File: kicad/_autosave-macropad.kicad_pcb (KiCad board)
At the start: 2 copper layers, 102 x 92 mm, 16 parts, among them J1 Conn_01x04_Socket, SW1 Kailh Choc, SW10 RotaryEncoder_Switch, SW11 RotaryEncoder_Switch, SW12 SW_Push, SW2 Kailh Choc, SW3 Kailh Choc, SW4 Kailh Choc, SW5 CherryMX, SW6 Kailh Choc, SW7 Kailh Choc, SW8 Kailh Choc, SW9 Kailh Choc, U1 Pico, U2 SKQUCAA010

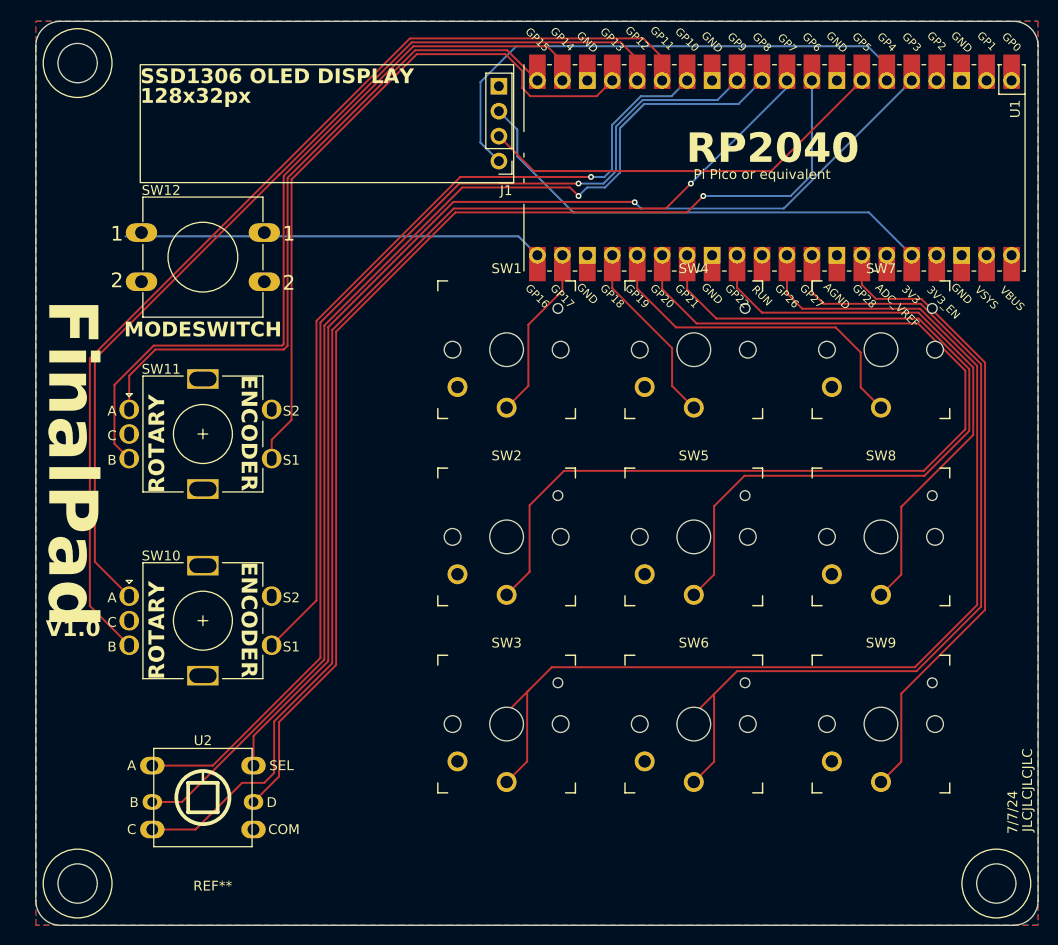
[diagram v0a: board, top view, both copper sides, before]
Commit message: updated
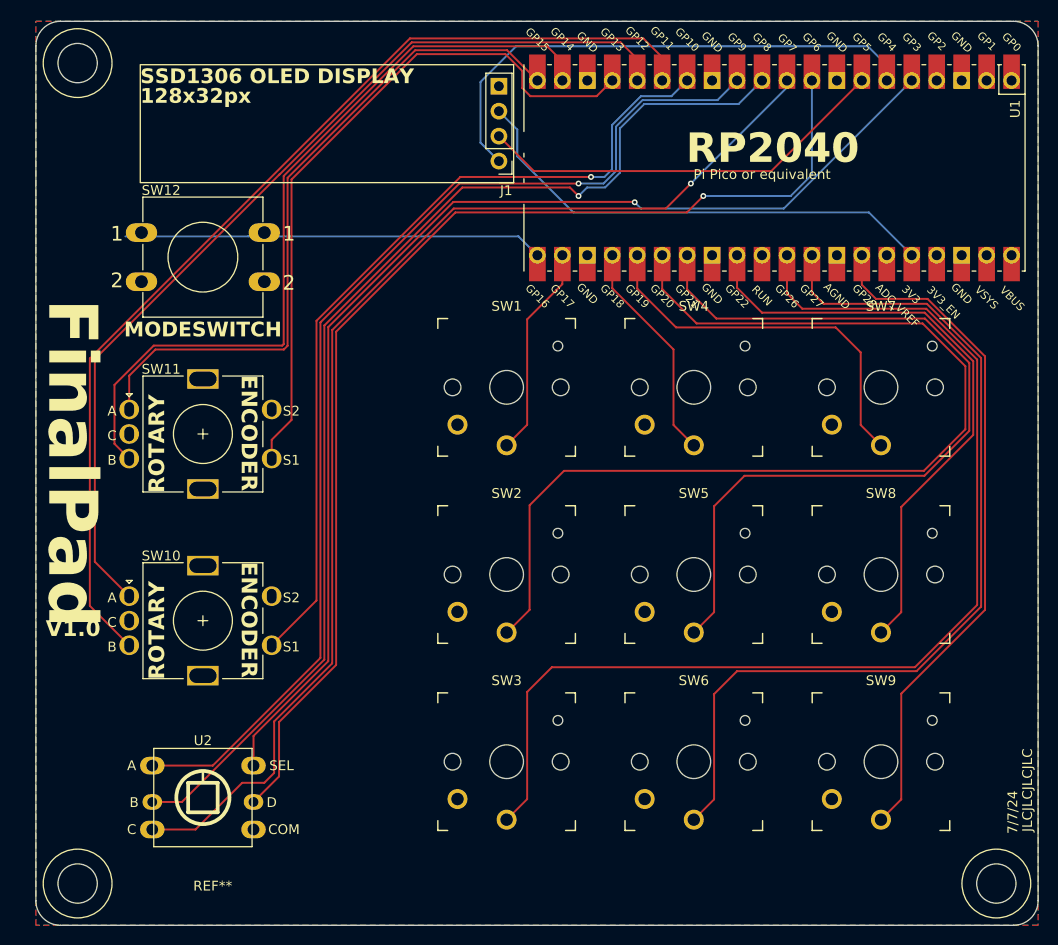
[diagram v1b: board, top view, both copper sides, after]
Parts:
- moved SW1 3.83 mm to (174.4, 77.8)
- moved SW2 3.83 mm to (174.4, 96.8)
- moved SW3 3.83 mm to (174.4, 115.8)
- moved SW4 3.83 mm to (193.5, 77.8)
- moved SW5 3.83 mm to (193.5, 96.8)
- moved SW6 3.83 mm to (193.5, 115.8)
- moved SW7 3.83 mm to (212.6, 77.8)
- moved SW8 3.83 mm to (212.6, 96.8)
- moved SW9 3.83 mm to (212.6, 115.8)
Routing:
- net Net-(U1-GPIO28_ADC2): track 65.9 -> 70.1 mm
- net Net-(U1-GPIO21): track 80.9 -> 85.1 mm
- net Net-(U1-GPIO19): track 35.3 -> 39.1 mm
- net Net-(U1-GPIO17): track 18.2 -> 21.7 mm
- net Net-(U1-GPIO20): track 102.2 -> 105.5 mm
- net Net-(U1-GPIO22): track 58.7 -> 61.9 mm
- net Net-(U1-GPIO18): track 19.7 -> 22.8 mm
- net Net-(U1-GPIO27_ADC1): track 92.3 -> 93.6 mm
